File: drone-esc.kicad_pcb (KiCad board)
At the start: 6 copper layers, 34 x 34 mm, 237 parts, among them J1 SM08B-SRSS-TB_LF__SN_, Q1 IRLHS6242, Q10 IRLHS6242, Q11 IRLHS6242, Q12 IRLHS6242, Q13 IRLHS6242, Q14 IRLHS6242, Q15 IRLHS6242, Q16 IRLHS6242, Q17 IRLHS6242, Q18 IRLHS6242, Q19 IRLHS6242, Q2 IRLHS6242, Q20 IRLHS6242, Q21 IRLHS6242, Q22 IRLHS6242, Q23 IRLHS6242, Q24 IRLHS6242, Q3 IRLHS6242, Q4 IRLHS6242, Q5 IRLHS6242, Q6 IRLHS6242, Q7 IRLHS6242, Q8 IRLHS6242, Q9 IRLHS6242, U10 DGD05473FNQ-7, U11 DGD05473FNQ-7, U12 AT32F421G8U7, U13 DGD05473FNQ-7, U14 DGD05473FNQ-7, U15 DGD05473FNQ-7, U16 AT32F421G8U7, U17 DGD05473FNQ-7, U18 DGD05473FNQ-7, U19 DGD05473FNQ-7, U2 INA186A3IDCKR, U20 AT32F421G8U7, U3 TLV76733DRVR, U4 TPS61023DRLR, U5 AT32F421G8U7, U6 DGD05473FNQ-7, U7 DGD05473FNQ-7, U8 DGD05473FNQ-7, U9 DGD05473FNQ-7

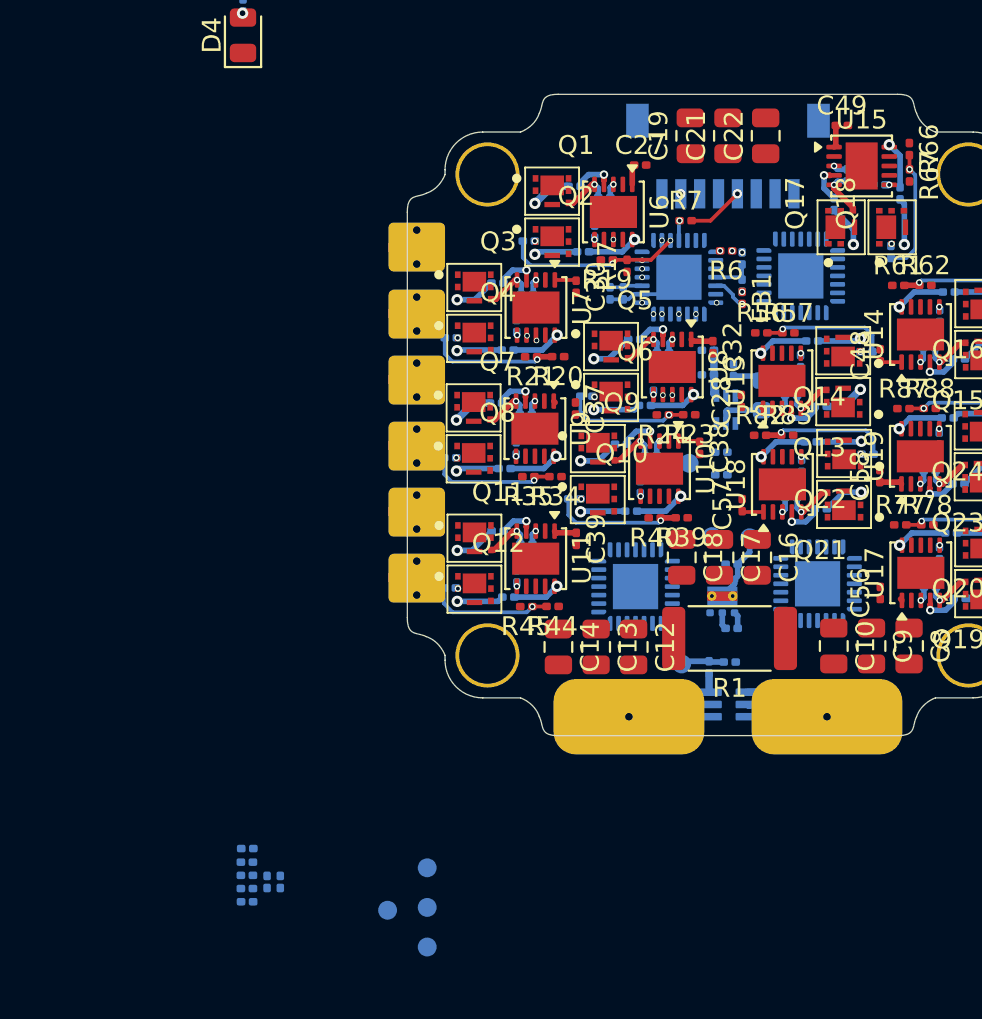
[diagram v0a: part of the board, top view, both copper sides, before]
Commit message: routed motor 1
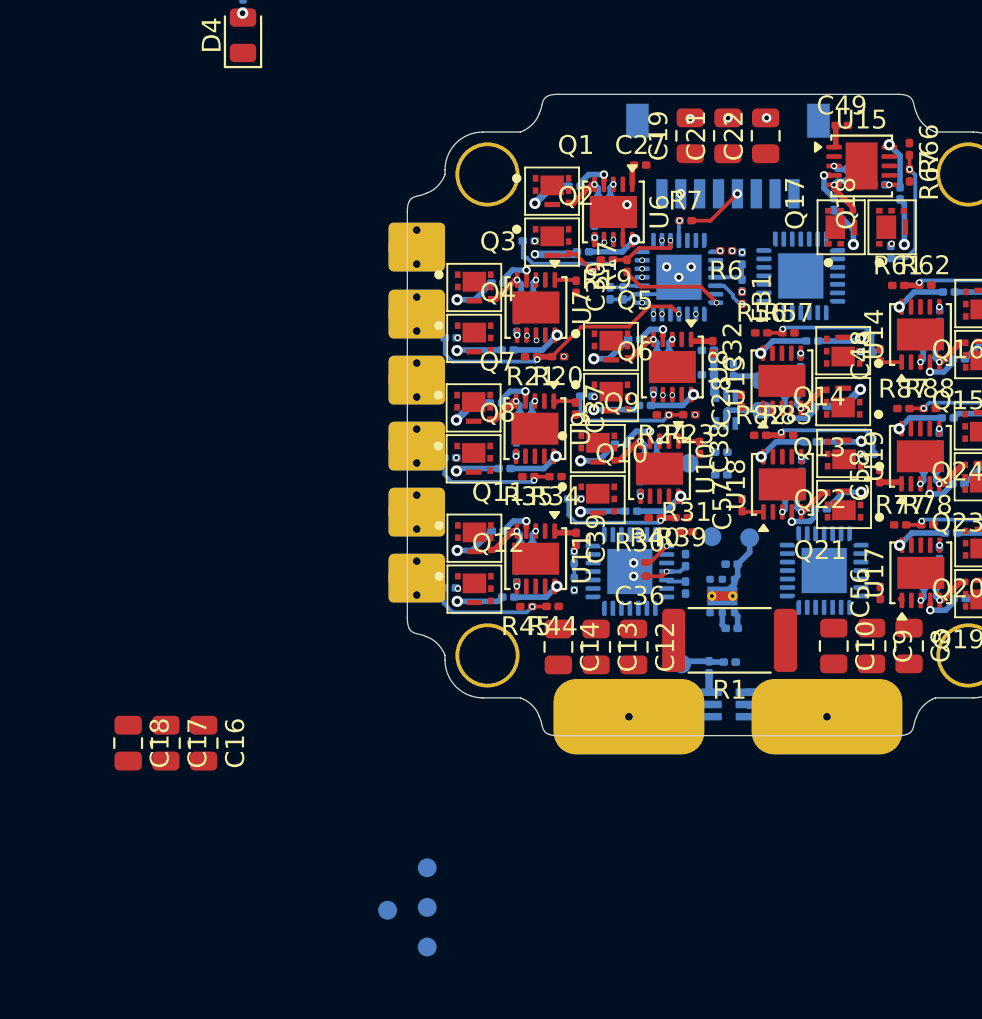
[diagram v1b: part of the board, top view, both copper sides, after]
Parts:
- C36, R30, R31: moved to F.Cu
- moved C16 31.0 mm to (117.2, 112.4)
- moved C17 31.0 mm to (115.2, 112.4)
- moved C18 31.0 mm to (113.2, 112.4)
- moved R31 28.7 mm to (142.8, 101.2)
- moved R26 28.6 mm to (142.8, 102.7), turned to -90 degrees
- moved FB2 28.6 mm to (142.8, 104.2), turned to 90 degrees
- moved C36 26.6 mm to (140.3, 103.5), turned to 180 degrees
- moved R30 26.2 mm to (140.3, 102.8), turned to 0 degrees
- moved C40 23.7 mm to (136.8, 102.5), turned to 90 degrees
- moved C41 22.2 mm to (136.8, 104.0)
- moved U12 0.85 mm to (139.8, 103.3)
- moved U20 0.78 mm to (150.1, 103.2)
- moved R1 0.10 mm to (145.1, 107.0)
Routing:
- net /ESC1/FBCOMMON: track 0.00 -> 22.4 mm, vias 1 -> 3
- net /ESC1/FBB: track 6.91 -> 14.9 mm
- net GND: track 11.5 -> 17.0 mm, vias 3 -> 15
- net /ESC1/A_HIGH: track 0.00 -> 2.42 mm, vias 1 -> 2
- net Net-(U12-NRST): track 0.00 -> 2.33 mm, vias 0 -> 1
- net Net-(U12-BOOT0): track 0.00 -> 1.47 mm, vias 0 -> 1
- net +5V: track 10.7 -> 11.9 mm
- net Net-(U12-VDDA): track 0.00 -> 1.03 mm
- net /ESC1/A_LOW: track 2.41 -> 3.41 mm
- net +3.3V: track 3.01 -> 3.79 mm
